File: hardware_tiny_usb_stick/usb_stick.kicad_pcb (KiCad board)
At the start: 2 copper layers, 40 x 15 mm, 27 parts, among them P1 USB_A, P2 CONN_02X05, P4 CONN_01X05, U1 AMS1117-3.3, U2 STM32F103CB, Y1 8M

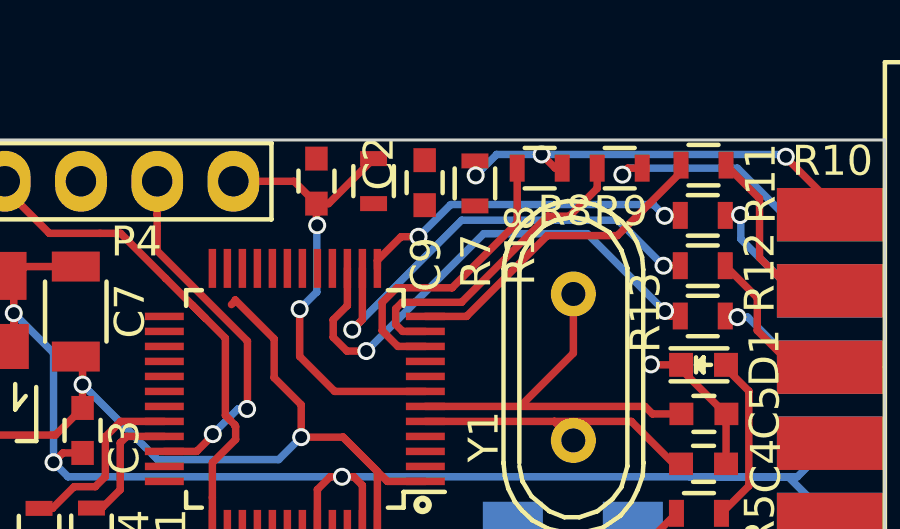
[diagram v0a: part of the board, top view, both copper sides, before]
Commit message: edit
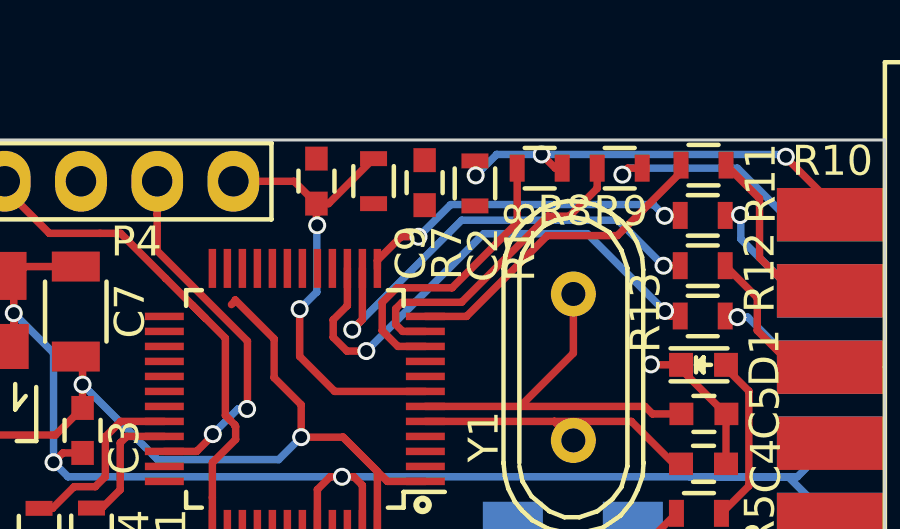
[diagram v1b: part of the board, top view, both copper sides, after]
